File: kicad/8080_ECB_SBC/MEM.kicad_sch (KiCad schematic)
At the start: 14 parts, among them U24 74LS00, U25 74LS32, U27 74LS32, U28 AS6C4008-55PCN, U29 SST39SF010, U30 74LS08

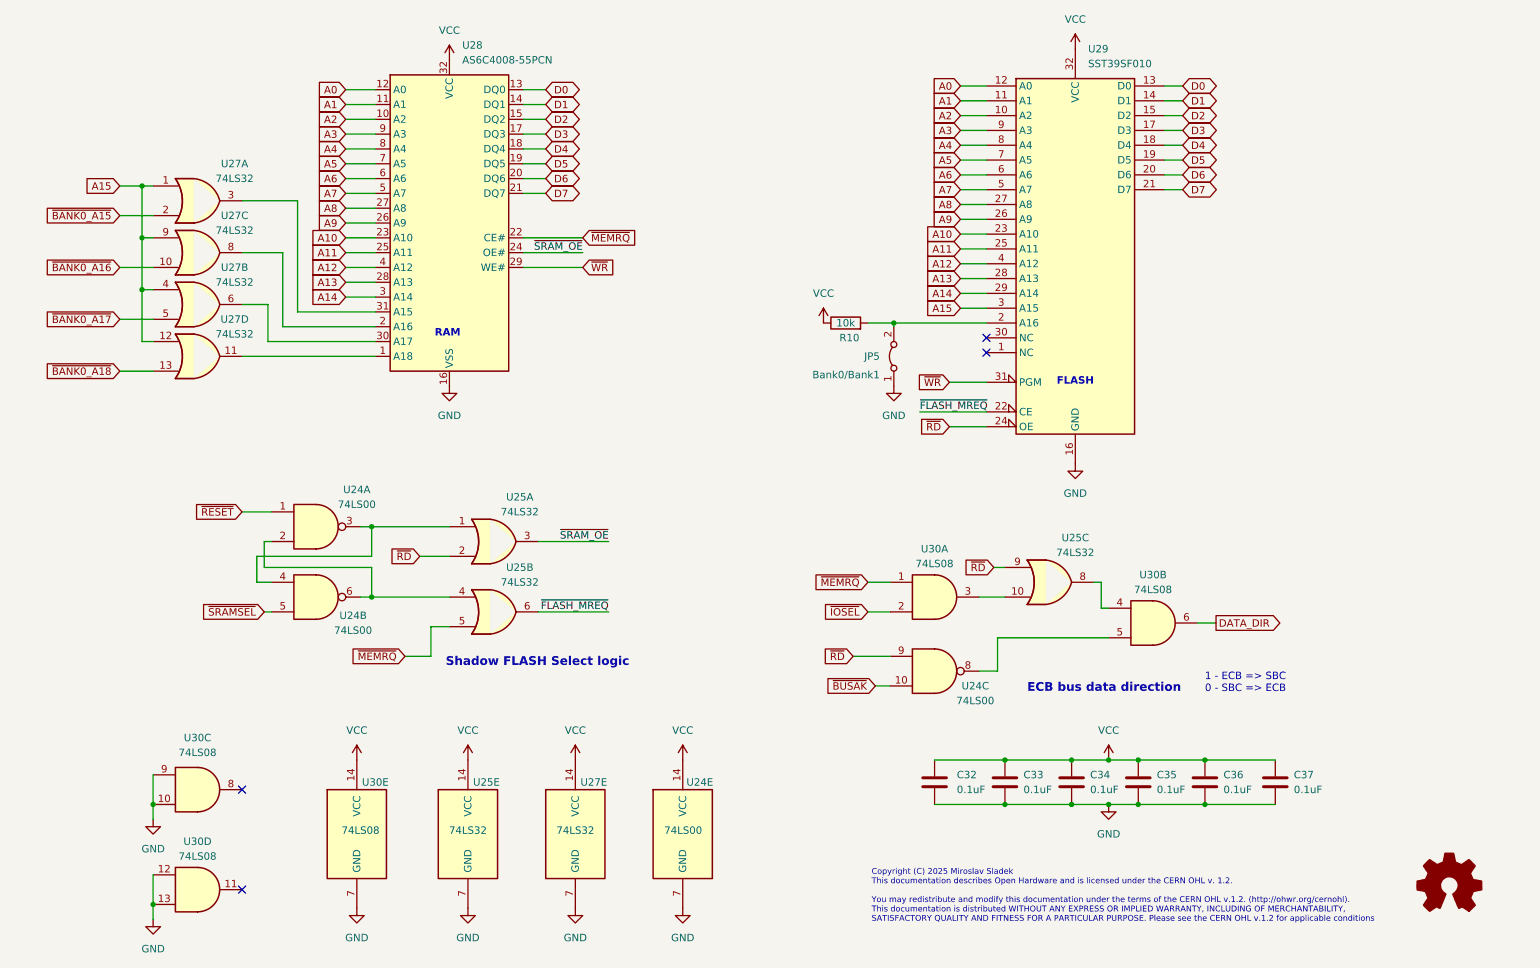
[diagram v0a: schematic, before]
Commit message: cleanup
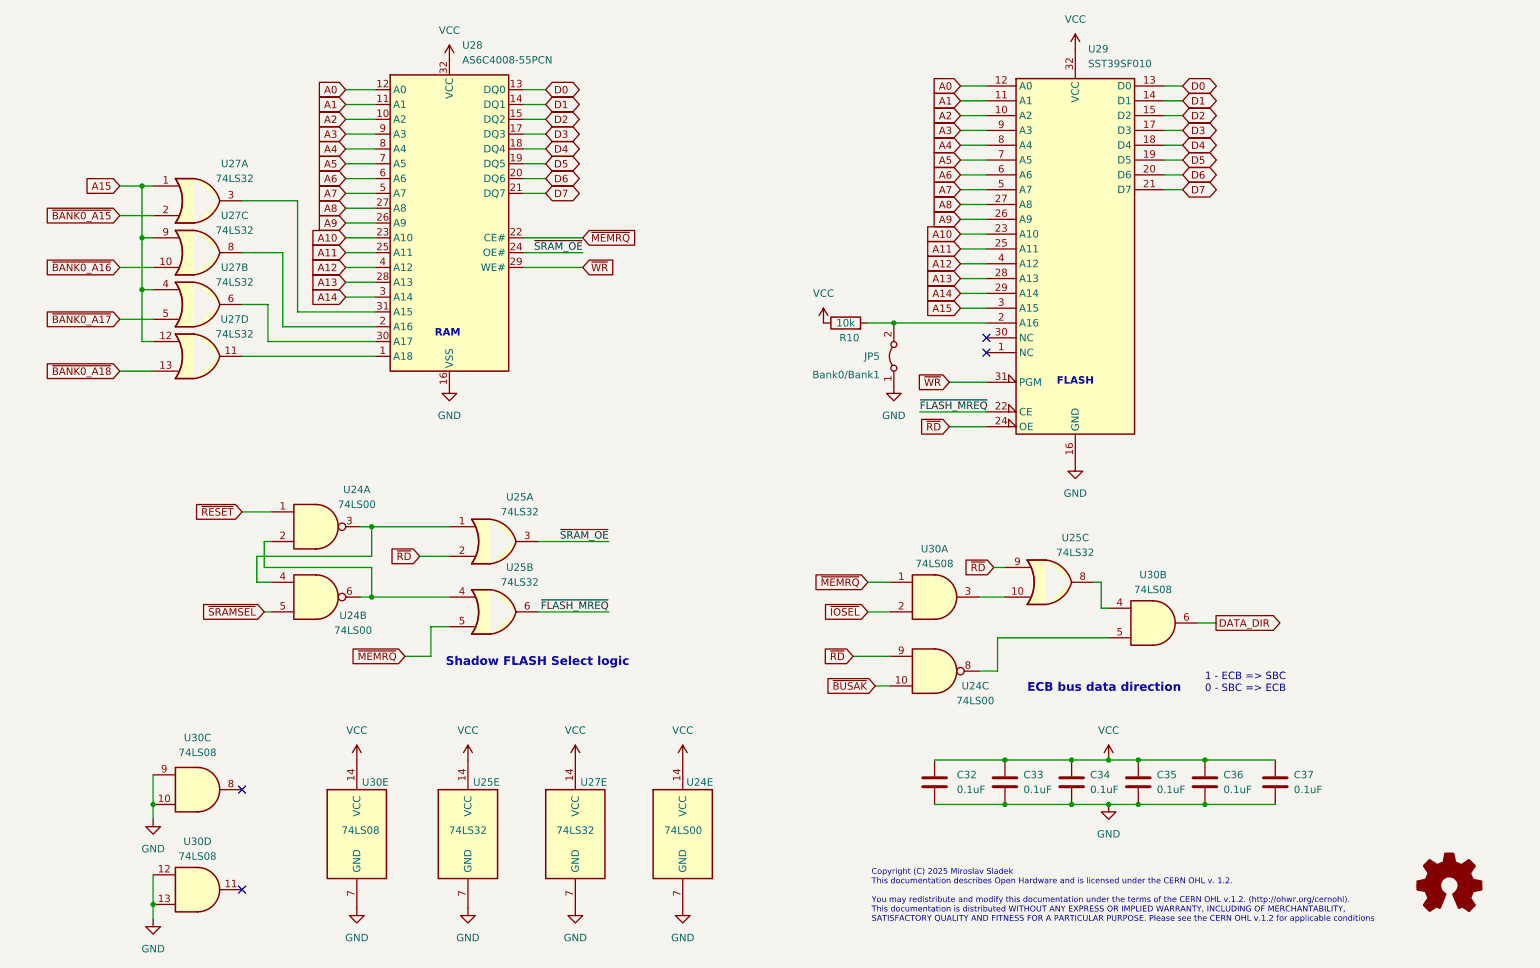
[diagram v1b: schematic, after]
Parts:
- R10: Mfr. No (none) -> CF18JT10K0; Nfr. No CF18JT10K0 -> (none)
